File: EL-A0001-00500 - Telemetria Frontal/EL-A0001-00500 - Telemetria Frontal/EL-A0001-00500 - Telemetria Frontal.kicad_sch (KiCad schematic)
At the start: 3 parts, among them J1 1-776087-1, U1 YAAJ_BluePill, U2 MP1584

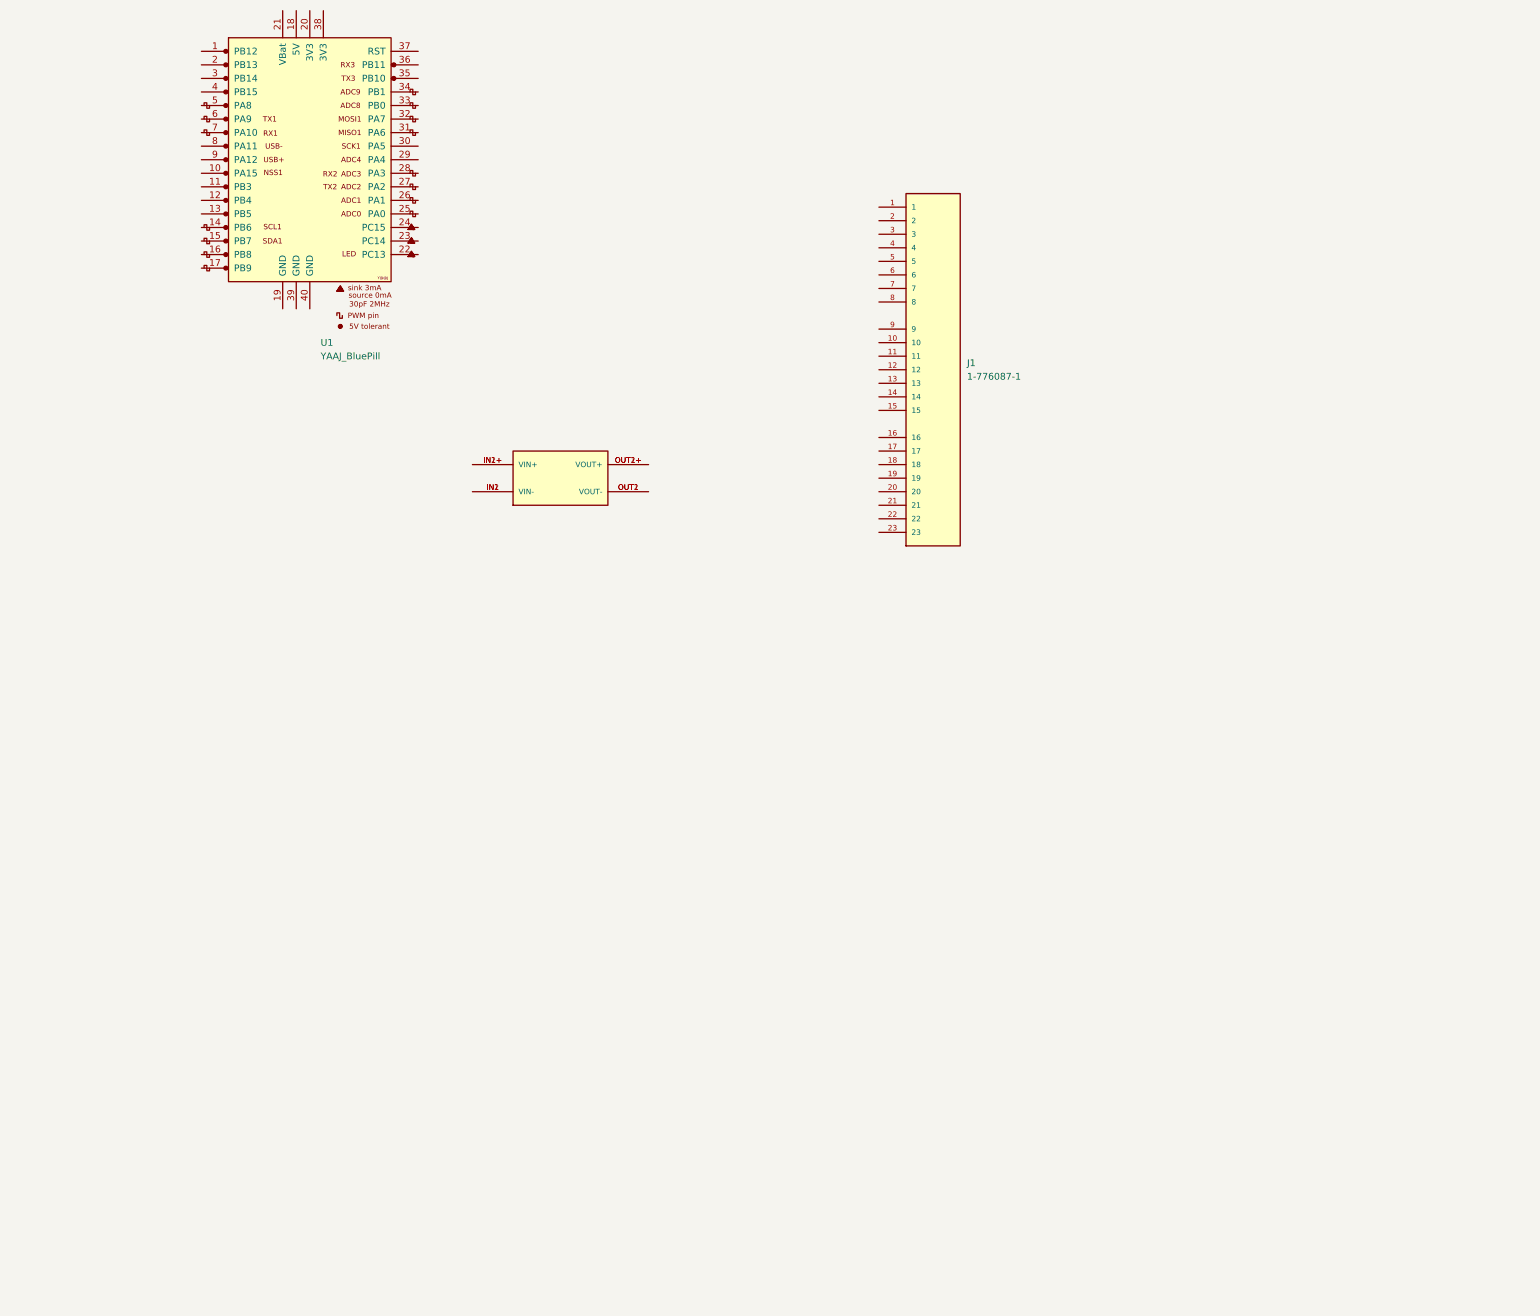
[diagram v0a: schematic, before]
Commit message: Telemetria frontal
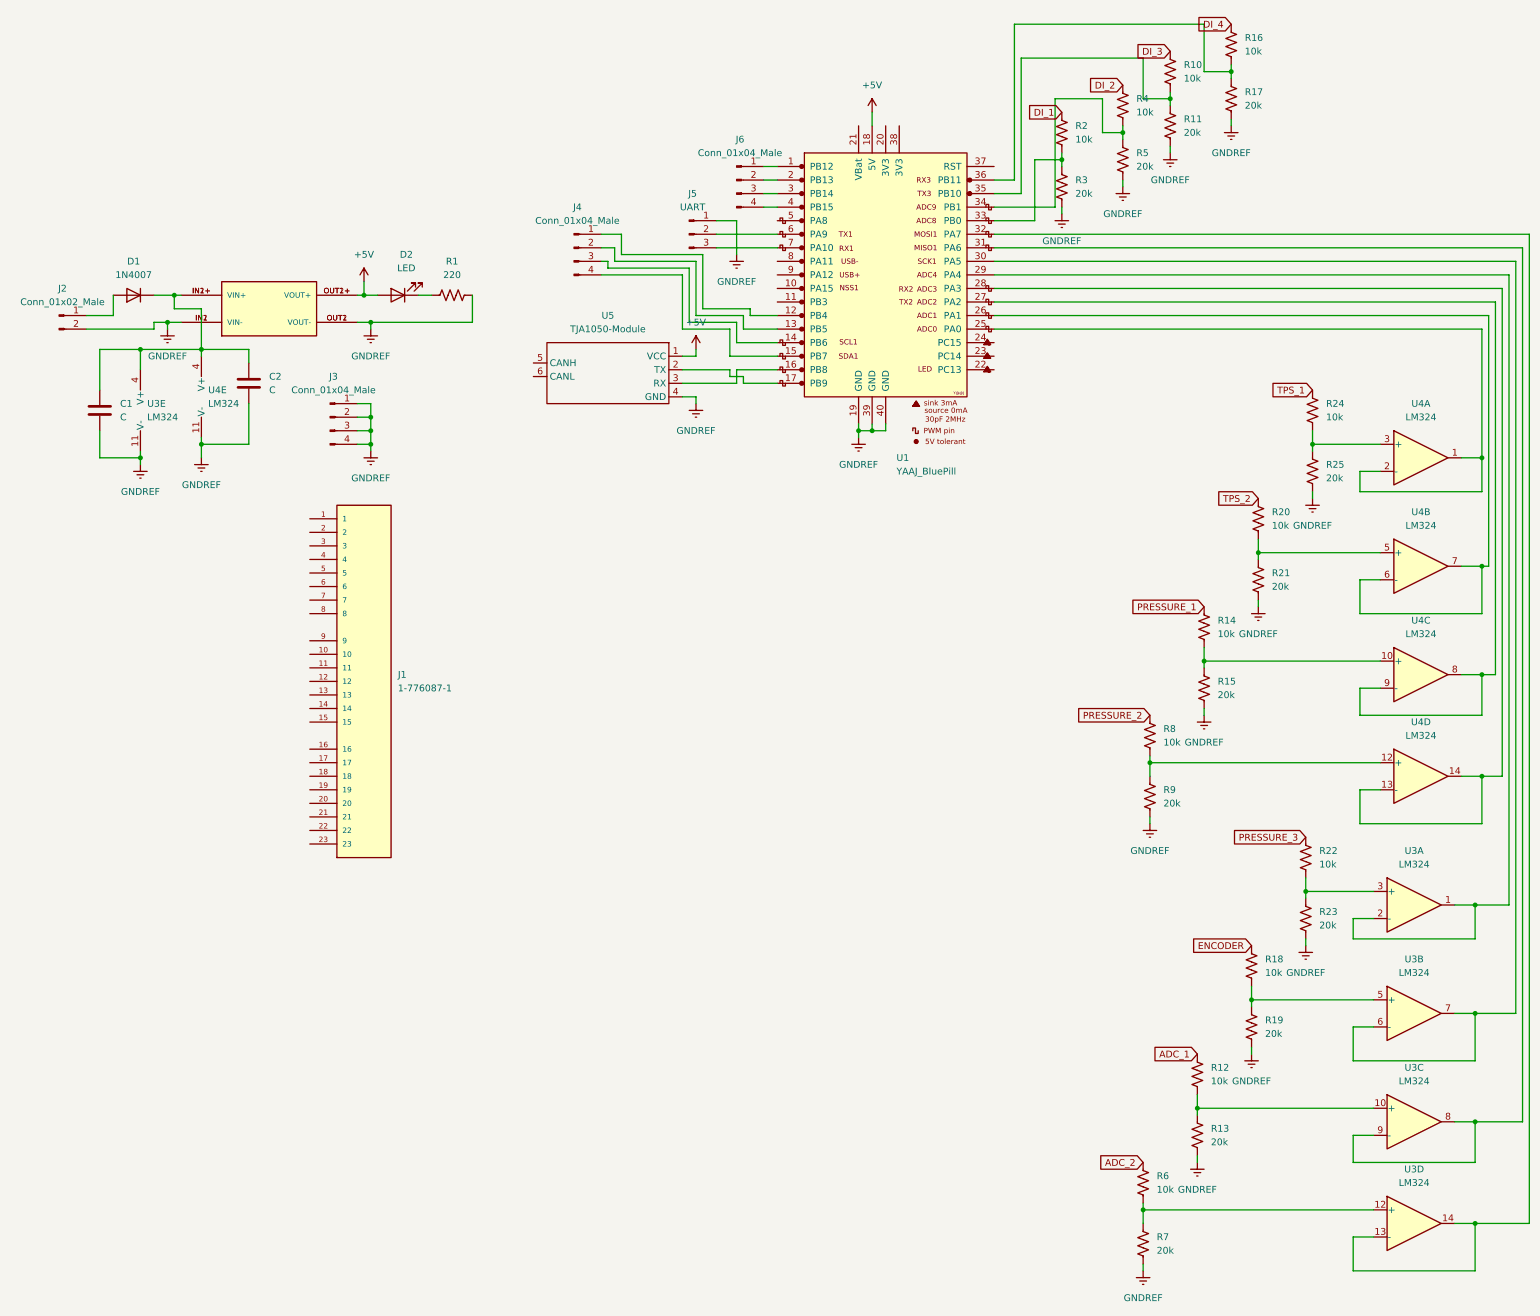
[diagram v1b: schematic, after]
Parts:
- added C1, C2: C, Capacitor_SMD:C_0805_2012Metric, symbol Device:C
- added D1: 1N4007, Diode_THT:D_DO-41_SOD81_P10.16mm_Horizontal, symbol Diode:1N4007
- added D2: LED, LED_THT:LED_D5.0mm, symbol Device:LED
- added J2: Conn_01x02_Male, Connector_PinHeader_2.54mm:PinHeader_1x02_P2.54mm_Vertical, symbol Connector:Conn_01x02_Male
- added J3, J4, J6: Conn_01x04_Male, Connector_PinHeader_2.54mm:PinHeader_1x04_P2.54mm_Vertical, symbol Connector:Conn_01x04_Male
- added J5: UART, Connector_PinHeader_2.54mm:PinHeader_1x03_P2.54mm_Vertical, symbol Connector:Conn_01x03_Male
- added R1: 220, Resistor_SMD:R_0805_2012Metric, symbol Device:R_US
- added R10, R12, R14, R16, R18, R2, R20, R22, R24, R4, R6, R8: 10k, Resistor_SMD:R_0805_2012Metric, symbol Device:R_US
- added R11, R13, R15, R17, R19, R21, R23, R25, R3, R5, R7, R9: 20k, Resistor_SMD:R_0805_2012Metric, symbol Device:R_US
- added U3, U4: LM324, Package_DIP:DIP-14_W7.62mm_LongPads, symbol Amplifier_Operational:LM324
- added U5: TJA1050-Module, Cheetah:TJA1050-Module, symbol Cheetah:TJA1050-Module
- U1: footprint STM32 Blue Pill:YAAJ_BluePill_1 -> STM32:YAAJ_BluePill_1
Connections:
- net at U1.1 (PB12): now also J6.1 (Pin_1)
- net at U1.12 (PB4): now also J4.1 (Pin_1)
- net at U1.13 (PB5): now also J4.2 (Pin_2)
- net at U1.14 (PB6): now also J4.3 (Pin_3)
- net at U1.15 (PB7): now also J4.4 (Pin_4)
- net at U1.16 (PB8): now also U5.3 (RX)
- net at U1.17 (PB9): now also U5.2 (TX)
- net +5V: now reaches U1.18 (5V)
- net +5V: now also U2.OUT1+ (VOUT+), U2.OUT2+ (VOUT+), D2.2 (A), U5.1 (VCC)
- net GNDREF: now reaches U1.19 (GND)
- net GNDREF: now also U1.39 (GND), U1.40 (GND), U2.IN1 (VIN-), U2.IN2 (VIN-), U2.OUT1 (VOUT-), U2.OUT2 (VOUT-), C1.2, C2.2, J2.2 (Pin_2), J3.1 (Pin_1), J3.2 (Pin_2), J3.3 (Pin_3), J3.4 (Pin_4), J5.1 (Pin_1), R1.2, R11.1, R13.1, R15.1, R17.1, R19.1, R21.1, R23.1, R25.1, R3.1, R5.1, R7.1, R9.1, U3.11 (V-), U4.11 (V-), U5.4 (GND)
- net at U1.2 (PB13): now also J6.2 (Pin_2)
- net at U1.25 (PA0): now also U4.1, U4.2 (-)
- net at U1.26 (PA1): now also U4.6 (-), U4.7
- net at U1.27 (PA2): now also U4.8, U4.9 (-)
- net at U1.28 (PA3): now also U4.13 (-), U4.14
- net at U1.29 (PA4): now also U3.1, U3.2 (-)
- net at U1.3 (PB14): now also J6.3 (Pin_3)
- net at U1.30 (PA5): now also U3.6 (-), U3.7
- net at U1.31 (PA6): now also U3.8, U3.9 (-)
- net at U1.32 (PA7): now also U3.13 (-), U3.14
- net at U1.33 (PB0): now also R2.1, R3.2
- net at U1.34 (PB1): now also R4.1, R5.2
- net at U1.35 (PB10): now also R10.1, R11.2
- net at U1.36 (PB11): now also R16.1, R17.2
- net at U1.4 (PB15): now also J6.4 (Pin_4)
- net at U1.6 (PA9): now also J5.2 (Pin_2)
- net at U1.7 (PA10): now also J5.3 (Pin_3)
- net at U2.IN1+ (VIN+), U2.IN2+ (VIN+): now also C1.1, C2.1, D1.1 (K), U3.4 (V+), U4.4 (V+)
- new net: R12.1, R13.2, U3.10 (+)
- new net: R14.1, R15.2, U4.10 (+)
- new net: R22.1, R23.2, U3.3 (+)
- new net: R6.1, R7.2, U3.12 (+)
- new net: R24.1, R25.2, U4.3 (+)
- new net: D2.1 (K), R1.1
- new net: R8.1, R9.2, U4.12 (+)
- new net: R18.1, R19.2, U3.5 (+)
- new net: R20.1, R21.2, U4.5 (+)
- new net: D1.2 (A), J2.1 (Pin_1)
- new net ADC_1: R12.2
- new net ADC_2: R6.2
- new net DI_1: R2.2
- new net DI_2: R4.2
- new net DI_3: R10.2
- new net DI_4: R16.2
- new net ENCODER: R18.2
- new net PRESSURE_1: R14.2
- new net PRESSURE_2: R8.2
- new net PRESSURE_3: R22.2
- new net TPS_1: R24.2
- new net TPS_2: R20.2
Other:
- moved on the sheet: J1, U1
